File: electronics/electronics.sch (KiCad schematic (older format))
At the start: 16 parts

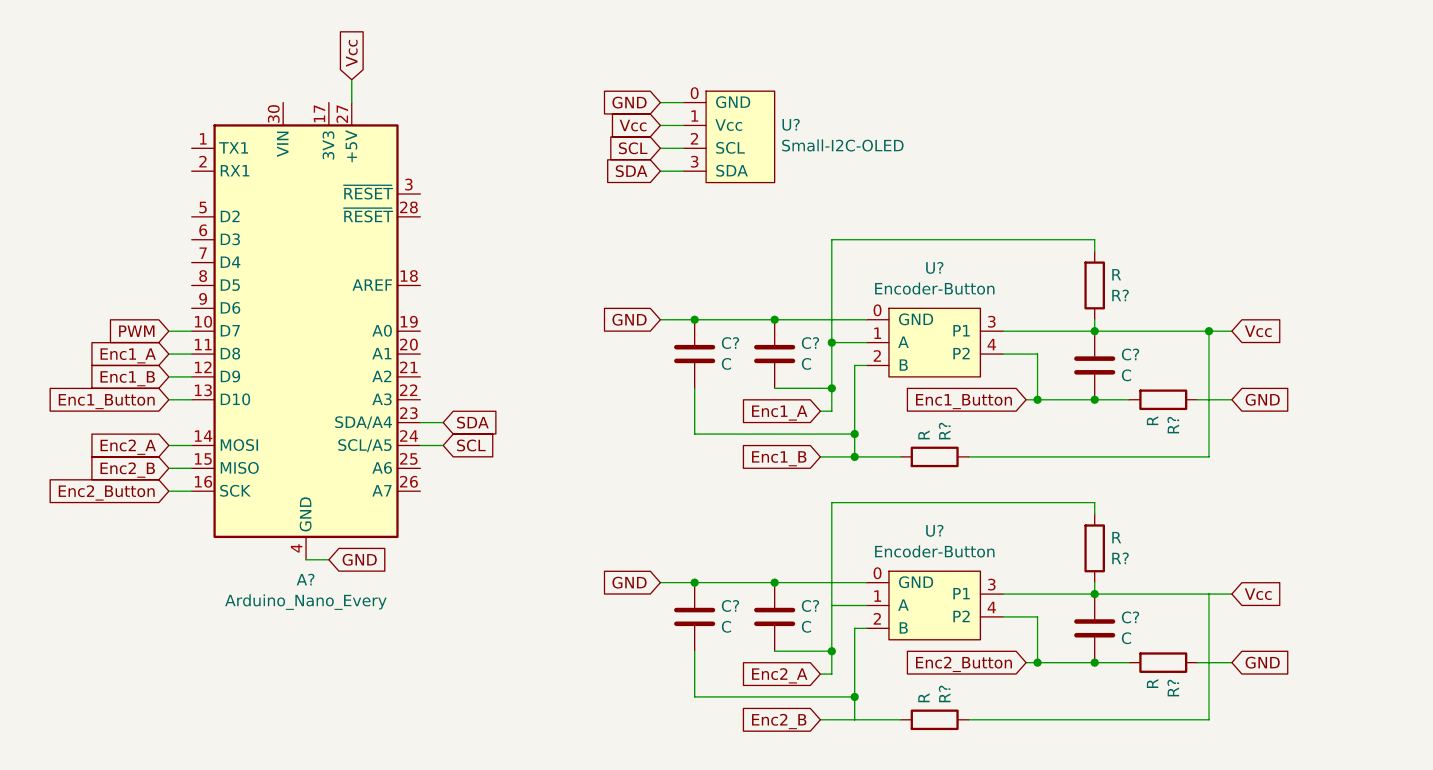
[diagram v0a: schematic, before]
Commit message: updates
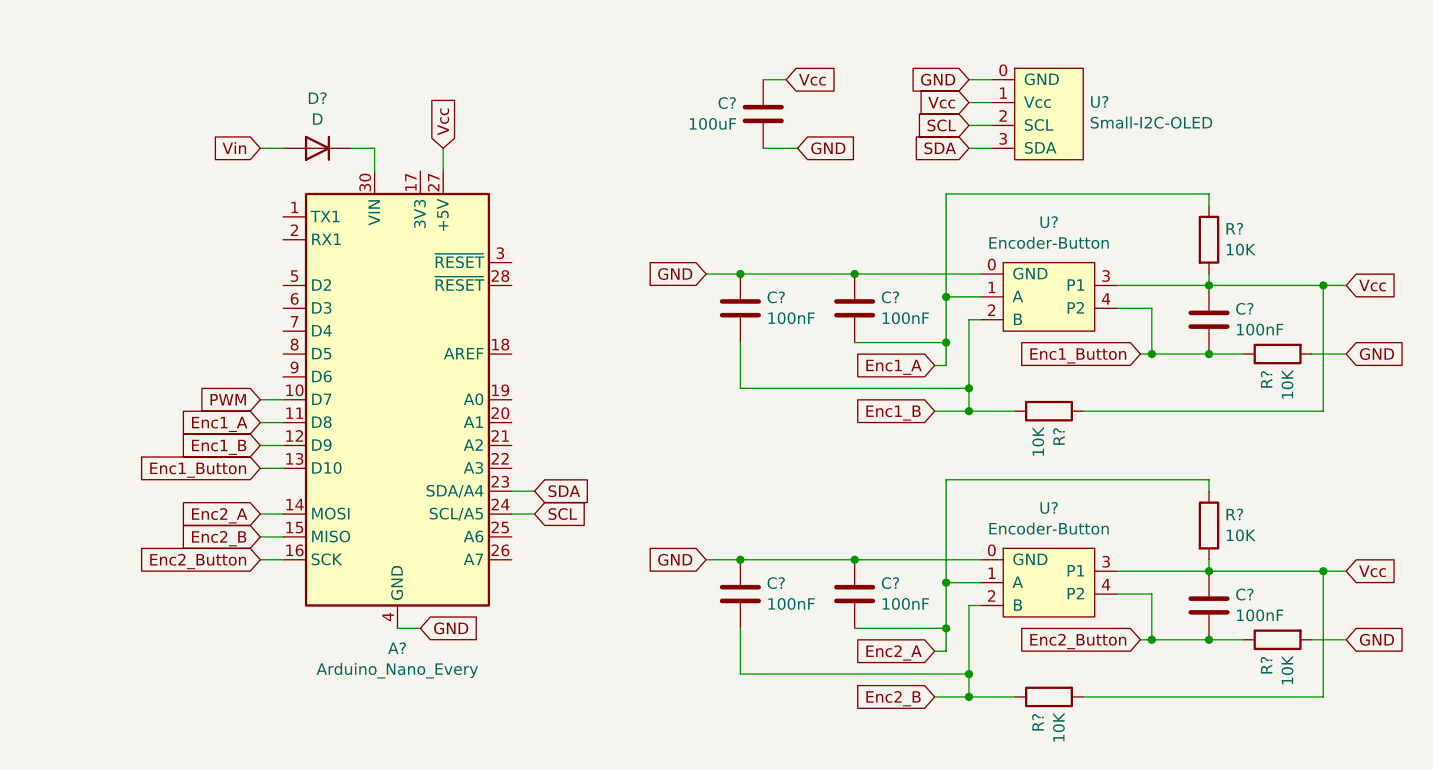
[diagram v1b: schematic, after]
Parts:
- added C?: 100uF, symbol Device:C
- added D?: D, symbol Device:D
- C? (x6): value C -> 100nF
- R? (x6): value R -> 10K
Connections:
- net Enc1_A: now also R?.1; no longer R?.2
- net Enc1_Button: now also R?.1; no longer R?.2
- net Enc2_A: now also R?.1; no longer R?.2
- net Enc2_B: now also R?.1; no longer R?.2
- net Enc2_Button: now also R?.1; no longer R?.2
- net GND: now also R?.2, R?.2, C?.2; no longer R?.1, R?.1
- net Vcc: now also R?.2, R?.2, R?.2, C?.1; no longer R?.1, R?.1
- net at A?.30 (VIN): now also D?.1 (K)
- new net Vin: D?.2 (A)
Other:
- moved on the sheet: A?, C?, R?, U?
